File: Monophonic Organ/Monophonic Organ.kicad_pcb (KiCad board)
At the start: 2 copper layers, 162.4 x 88.9 mm, 106 parts, among them IC1 NE555DR, IC2 NE555DR, IC3 HEF4069UBT,653, IC4 LT1782CS5#TRMPBF, J1 Speaker, Q1 Si2338DS-T1-GE3, Q2 BC858, Q3 Si2338DS-T1-GE3, Q4 BC848, Q5 BC858, Q6 BC848

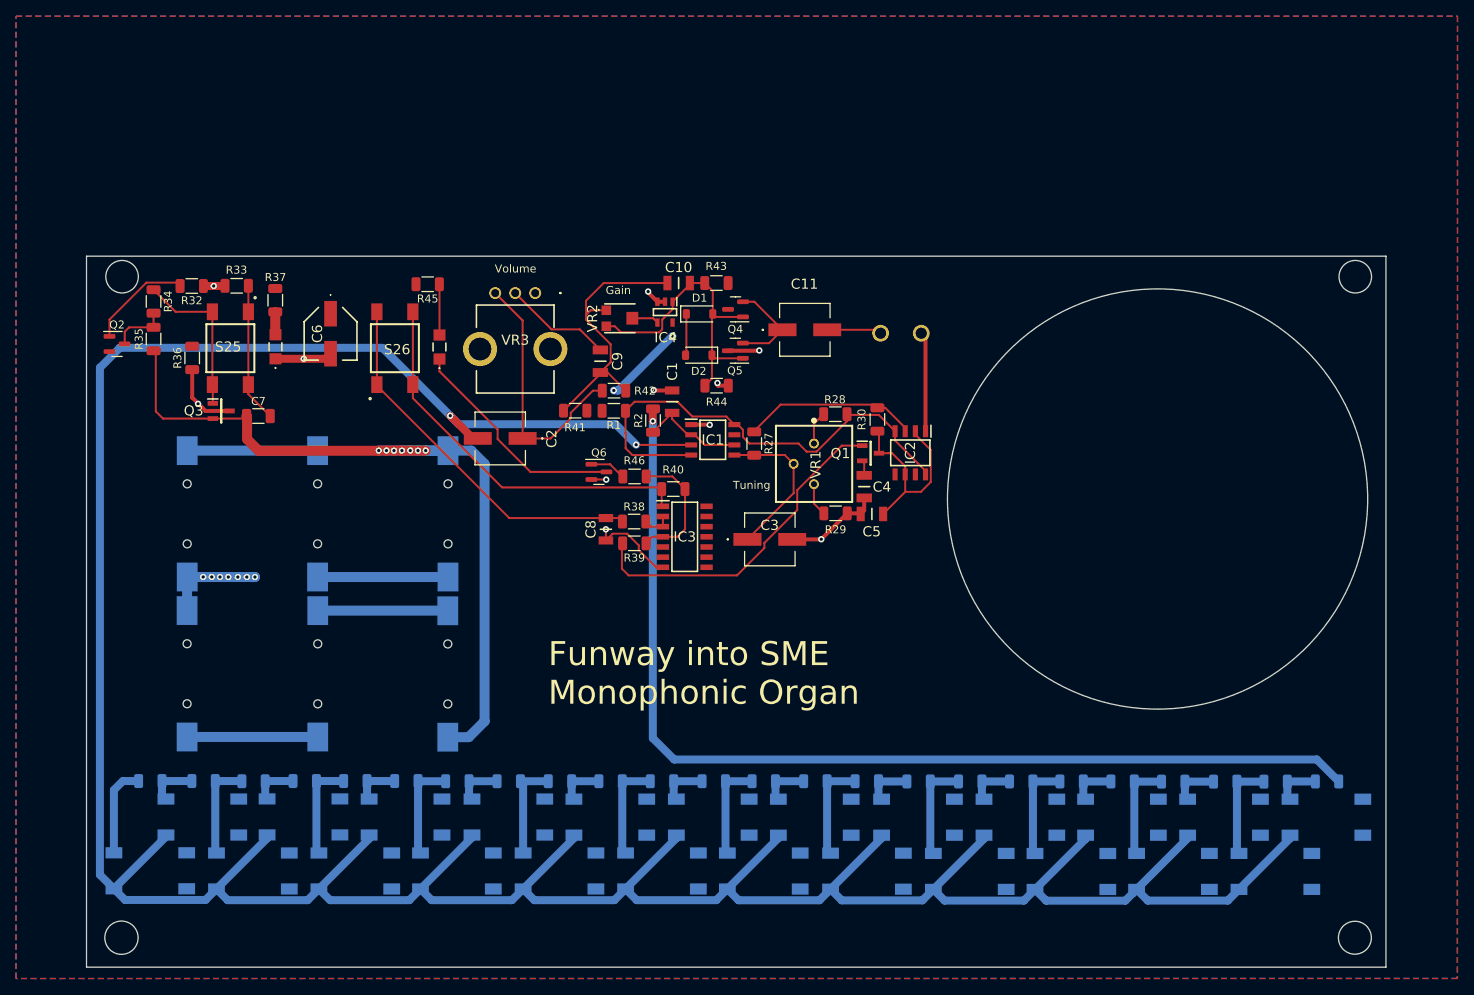
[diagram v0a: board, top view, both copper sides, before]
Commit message: Fixed mistake on organ pcb
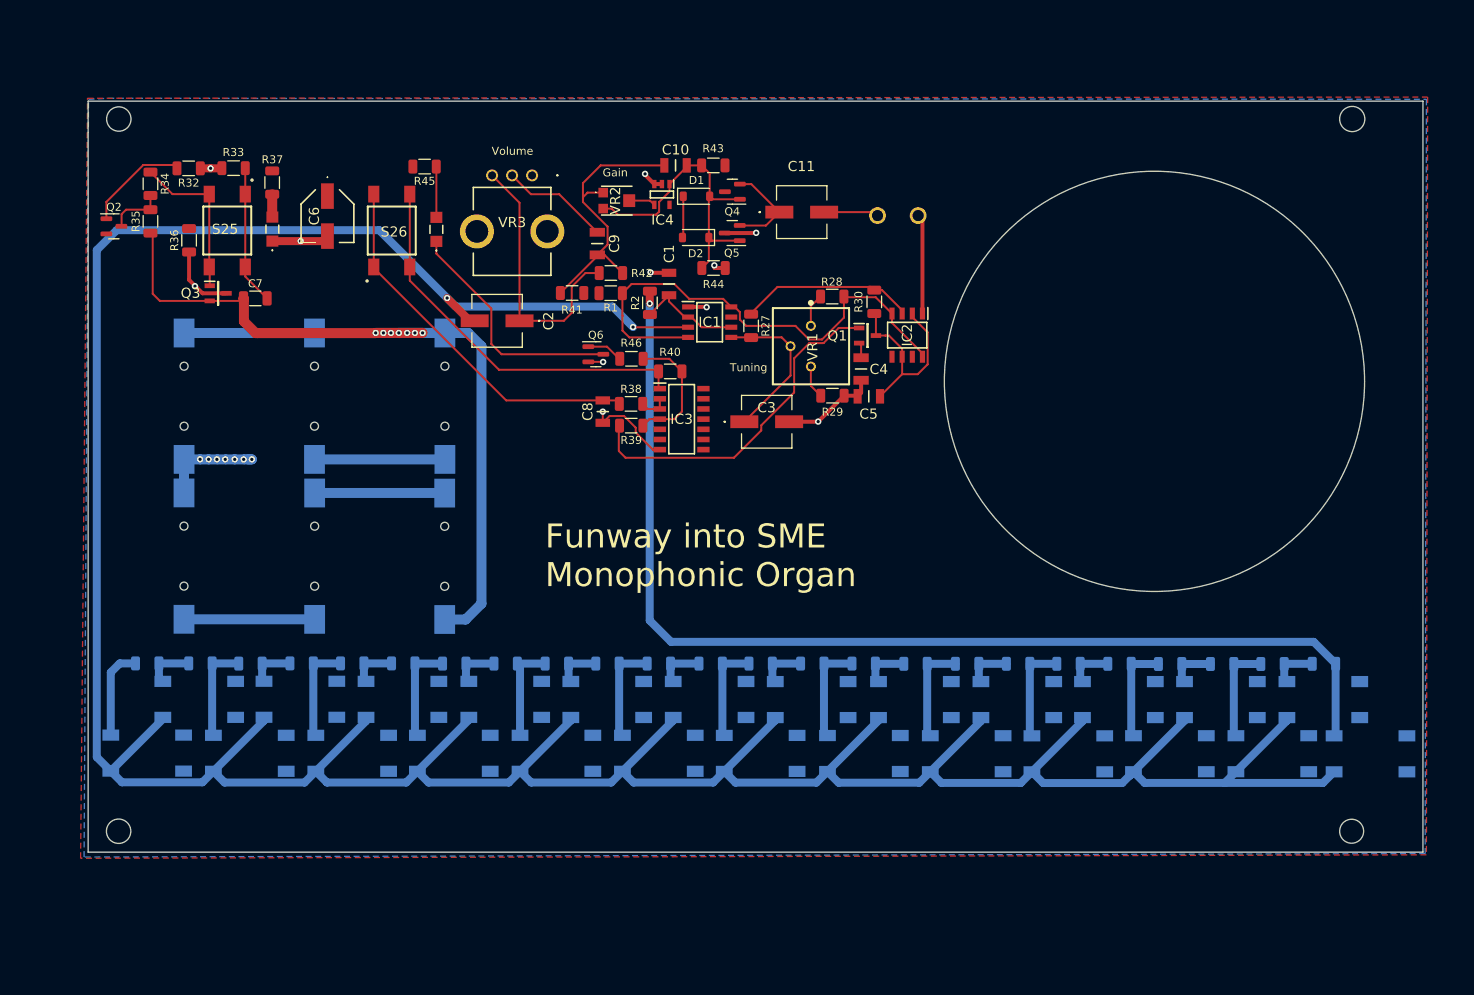
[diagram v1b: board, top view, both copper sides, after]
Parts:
- added S27: FSM4JSMATR, SamacSys_Parts:FSM4JSMATR, B.Cu at (207.4, 120.6)
- moved B4 14.7 mm to (91.7, 95.9)
- moved B5 14.7 mm to (75.4, 95.9)
- moved C5 14.7 mm to (144.7, 75.9)
- moved C8 14.7 mm to (111.4, 77.8)
- moved Q1 14.7 mm to (144.5, 68.3)
- moved R10 14.7 mm to (157.0, 109.3)
- moved R11 14.7 mm to (150.5, 109.3)
- moved R2 14.7 mm to (117.3, 64.2)
- moved R29 14.7 mm to (140.2, 75.8)
- moved R3 14.7 mm to (201.6, 109.3)
- moved R34 14.7 mm to (54.9, 49.3)
- moved R36 14.7 mm to (59.7, 56.4)
- moved R39 14.7 mm to (115.0, 79.6)
- moved R46 14.7 mm to (115.0, 71.2)
- moved R7 14.7 mm to (176.0, 109.3)
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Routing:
- net PROBE: track 416.6 -> 430.8 mm
- net 9V: track 22.9 -> 12.8 mm, vias 9 -> 7
- net Net-(R2-Pad2): track 129.2 -> 138.3 mm
- net Net-(LED2-K): track 28.3 -> 30.2 mm
- net Net-(IC1-VCC): track 60.8 -> 62.4 mm
- net AUDIO GND: track 32.4 -> 33.9 mm
- net VIBRATO: track 42.4 -> 43.4 mm
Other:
- board size 162.4 x 88.9 mm -> 166.9 x 93.9 mm
